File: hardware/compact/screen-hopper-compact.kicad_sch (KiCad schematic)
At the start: 11 parts, among them J1 USB_A_Host, J2 USB_C_Host, U1 6N137

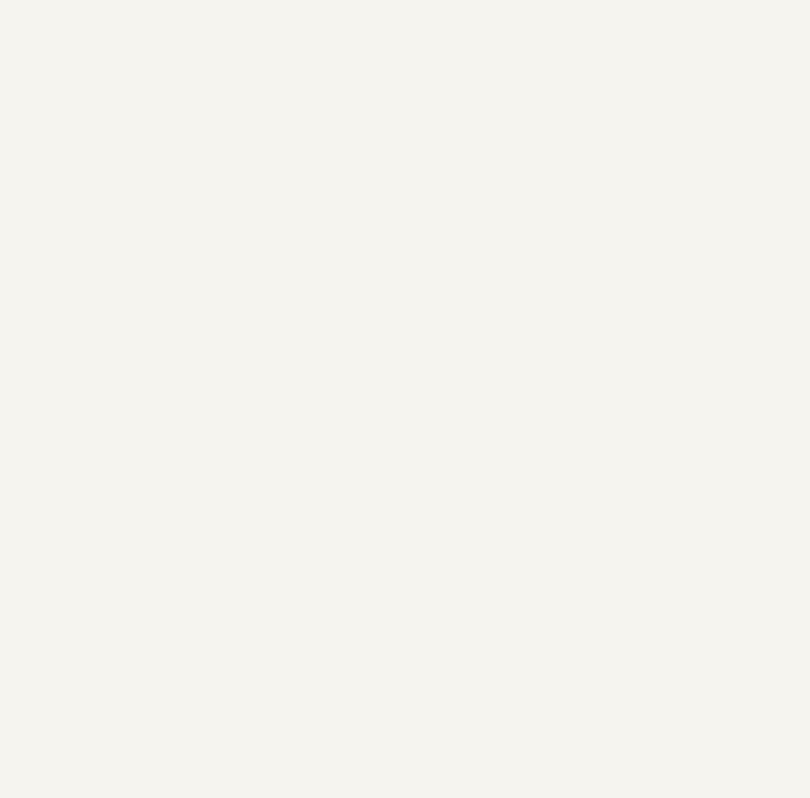
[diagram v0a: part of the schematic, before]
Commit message: feat: hardware board designs
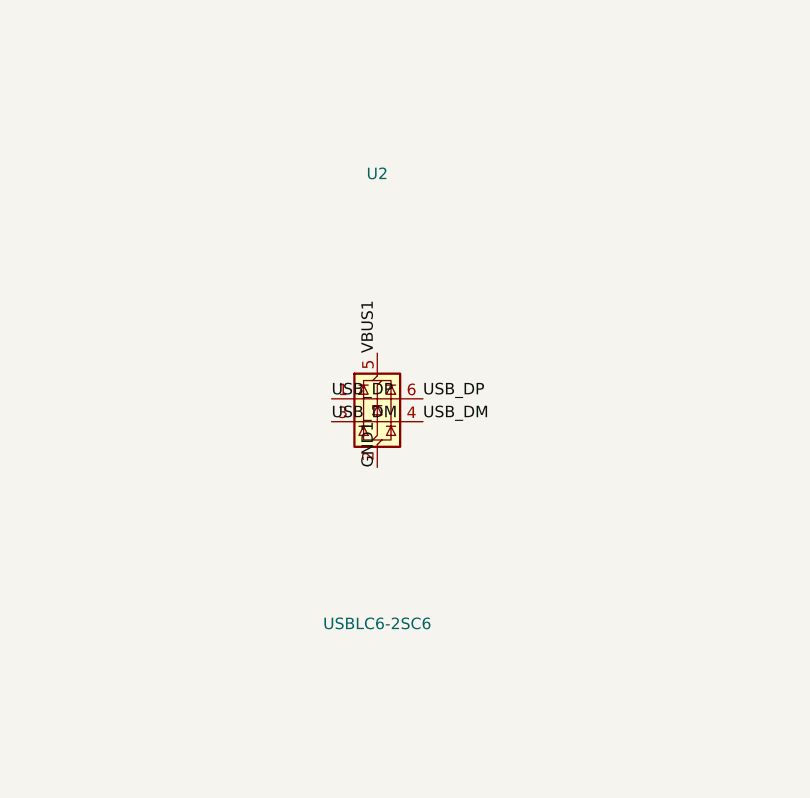
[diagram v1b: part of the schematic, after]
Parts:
- added U2: USBLC6-2SC6, Package_TO_SOT_SMD:SOT-23-6, symbol Power_Protection:USBLC6-2SC6
- J1: footprint Connector_USB:USB_A_Connfly_DS1095 -> Connector_USB:USB_A_TE_292303-7_Horizontal
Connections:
- net GND1: now also U2.2 (GND)
- net USB_DM: now also U2.3 (I/O2), U2.4 (I/O2)
- net USB_DP: now also U2.1 (I/O1), U2.6 (I/O1)
- net VBUS1: now also U2.5 (VBUS)
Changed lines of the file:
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@@
 		(instances
 			(project "screen-hopper"
-				(path "/1ca3d3a5-c661-41a7-ad19-cf03fba76b71"
+				(path "/e4afde65-c9ae-401d-b381-77b0abf5f55b"
 					(reference "A1")
 					(unit 1)
@@
 		(instances
 			(project "screen-hopper"
-				(path "/1ca3d3a5-c661-41a7-ad19-cf03fba76b71"
+				(path "/e4afde65-c9ae-401d-b381-77b0abf5f55b"
 					(reference "A2")
 					(unit 1)
@@
 		(instances
 			(project "screen-hopper"
-				(path "/1ca3d3a5-c661-41a7-ad19-cf03fba76b71"
+				(path "/e4afde65-c9ae-401d-b381-77b0abf5f55b"
 					(reference "A3")
 					(unit 1)
@@
 		(instances
 			(project "screen-hopper"
-				(path "/1ca3d3a5-c661-41a7-ad19-cf03fba76b71"
+				(path "/e4afde65-c9ae-401d-b381-77b0abf5f55b"
 					(reference "U1")
 					(unit 1)
@@
 		(instances
 			(project "screen-hopper"
-				(path "/1ca3d3a5-c661-41a7-ad19-cf03fba76b71"
+				(path "/e4afde65-c9ae-401d-b381-77b0abf5f55b"
 					(reference "R1")
 					(unit 1)
@@
 		(instances
 			(project "screen-hopper"
-				(path "/1ca3d3a5-c661-41a7-ad19-cf03fba76b71"
+				(path "/e4afde65-c9ae-401d-b381-77b0abf5f55b"
 					(reference "R2")
 					(unit 1)
@@
 		(instances
 			(project "screen-hopper"
-				(path "/1ca3d3a5-c661-41a7-ad19-cf03fba76b71"
+				(path "/e4afde65-c9ae-401d-b381-77b0abf5f55b"
 					(reference "C1")
 					(unit 1)
@@
 			(effects (font (size 1.27 1.27)))
 		)
-		(property "Footprint" "Connector_USB:USB_A_Connfly_DS1095"
+		(property "Footprint" "Connector_USB:USB_A_TE_292303-7_Horizontal"
 			(at 90.00 250.00 0)
 			(effects (font (size 1.27 1.27)) (hide yes))
@@
 		(instances
 			(project "screen-hopper"
-				(path "/1ca3d3a5-c661-41a7-ad19-cf03fba76b71"
+				(path "/e4afde65-c9ae-401d-b381-77b0abf5f55b"
 					(reference "J1")
 					(unit 1)
@@
 		(instances
 			(project "screen-hopper"
-				(path "/1ca3d3a5-c661-41a7-ad19-cf03fba76b71"
+				(path "/e4afde65-c9ae-401d-b381-77b0abf5f55b"
 					(reference "R3")
 					(unit 1)
@@
 		(instances
 			(project "screen-hopper"
-				(path "/1ca3d3a5-c661-41a7-ad19-cf03fba76b71"
+				(path "/e4afde65-c9ae-401d-b381-77b0abf5f55b"
 					(reference "R4")
 					(unit 1)
@@
 		(instances
 			(project "screen-hopper"
-				(path "/1ca3d3a5-c661-41a7-ad19-cf03fba76b71"
+				(path "/e4afde65-c9ae-401d-b381-77b0abf5f55b"
 					(reference "J2")
+					(unit 1)
+				)
+			)
+		)
+	)
+	(symbol
+		(lib_id "Power_Protection:USBLC6-2SC6")
+		(at 190.00 320.00 0)
+		(unit 1)
+		(exclude_from_sim no)
+		(in_bom yes)
+		(on_board yes)
+		(dnp no)
+		(property "Reference" "U2"
+			(at 190.00 295.00 0)
+			(effects (font (size 1.27 1.27)))
+		)
+		(property "Value" "USBLC6-2SC6"
+			(at 190.00 345.00 0)
+			(effects (font (size 1.27 1.27)))
+		)
+		(property "Footprint" "Package_TO_SOT_SMD:SOT-23-6"
+			(at 190.00 320.00 0)
+			(effects (font (size 1.27 1.27)) (hide yes))
+		)
+		(pin "1"
+		)
+		(pin "2"
+		)
+		(pin "3"
+		)
+		(pin "4"
+		)
+		(pin "5"
+		)
+		(pin "6"
+		)
+		(instances
+			(project "screen-hopper"
+				(path "/e4afde65-c9ae-401d-b381-77b0abf5f55b"
+					(reference "U2")
 					(unit 1)
 				)
@@
 		(effects (font (size 1.27 1.27)) (justify left bottom))
 	)
+	(label "VBUS1"
+		(at 190.00 314.92 270)
+		(effects (font (size 1.27 1.27)) (justify left bottom))
+	)
 	(label "GND1"
 		(at 190.00 195.56 90)
@@
 	(label "GND1"
 		(at 82.38 362.86 90)
+		(effects (font (size 1.27 1.27)) (justify left bottom))
+	)
+	(label "GND1"
+		(at 190.00 327.62 90)
 		(effects (font (size 1.27 1.27)) (justify left bottom))
 	)
@@
 		(effects (font (size 1.27 1.27)) (justify left bottom))
 	)
+	(label "USB_DM"
+		(at 184.92 322.54 0)
+		(effects (font (size 1.27 1.27)) (justify left bottom))
+	)
+	(label "USB_DM"
+		(at 195.08 322.54 180)
+		(effects (font (size 1.27 1.27)) (justify left bottom))
+	)
 	(label "USB_DP"
 		(at 97.62 250.00 180)
@@
 		(effects (font (size 1.27 1.27)) (justify left bottom))
 	)
+	(label "USB_DP"
+		(at 184.92 320.00 0)
+		(effects (font (size 1.27 1.27)) (justify left bottom))
+	)
+	(label "USB_DP"
+		(at 195.08 320.00 180)
+		(effects (font (size 1.27 1.27)) (justify left bottom))
+	)

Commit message: feat: hardware board designs
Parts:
- A1, A2, A3: MPN (none) -> SC1631; Manufacturer (none) -> Raspberry Pi
- J1: MPN (none) -> 292303-7; Manufacturer (none) -> TE Connectivity
- J2: MPN (none) -> TYPE-C-31-M-12; Manufacturer (none) -> HRO
- R1: MPN (none) -> RC0805JR-07470RL; Manufacturer (none) -> Yageo
- R2: MPN (none) -> RC0805FR-07680RL; Manufacturer (none) -> Yageo
- R3, R4: MPN (none) -> AC0805FR-0756KL; Manufacturer (none) -> Yageo
- U1: MPN (none) -> 6N137SM; Manufacturer (none) -> onsemi
- U2: MPN (none) -> USBLC6-2SC6; Manufacturer (none) -> STMicroelectronics
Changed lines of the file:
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@@
+			(effects (font (size 1.27 1.27)) (hide yes))
+		)
+		(property "MPN" "SC1631"
+			(at 190.00 160.00 0)
+			(effects (font (size 1.27 1.27)) (hide yes))
+		)
+		(property "Manufacturer" "Raspberry Pi"
+			(at 190.00 160.00 0)
 			(effects (font (size 1.27 1.27)) (hide yes))
 		)
@@
 		(instances
 			(project "screen-hopper"
-				(path "/546f9845-45df-437b-a8f0-1d6148817de3"
+				(path "/468433d7-c8e3-4031-b0d4-1b453175f0b2"
 					(reference "A1")
 					(unit 1)
@@
 			(effects (font (size 1.27 1.27)) (hide yes))
 		)
+		(property "MPN" "SC1631"
+			(at 90.00 160.00 0)
+			(effects (font (size 1.27 1.27)) (hide yes))
+		)
+		(property "Manufacturer" "Raspberry Pi"
+			(at 90.00 160.00 0)
+			(effects (font (size 1.27 1.27)) (hide yes))
+		)
 		(pin "1"
 		)
@@
 		(instances
 			(project "screen-hopper"
-				(path "/546f9845-45df-437b-a8f0-1d6148817de3"
+				(path "/468433d7-c8e3-4031-b0d4-1b453175f0b2"
 					(reference "A2")
 					(unit 1)
@@
 			(effects (font (size 1.27 1.27)) (hide yes))
 		)
+		(property "MPN" "SC1631"
+			(at 290.00 160.00 0)
+			(effects (font (size 1.27 1.27)) (hide yes))
+		)
+		(property "Manufacturer" "Raspberry Pi"
+			(at 290.00 160.00 0)
+			(effects (font (size 1.27 1.27)) (hide yes))
+		)
 		(pin "1"
 		)
@@
 		(instances
 			(project "screen-hopper"
-				(path "/546f9845-45df-437b-a8f0-1d6148817de3"
+				(path "/468433d7-c8e3-4031-b0d4-1b453175f0b2"
 					(reference "A3")
 					(unit 1)
@@
 			(effects (font (size 1.27 1.27)) (hide yes))
 		)
+		(property "MPN" "6N137SM"
+			(at 185.00 70.00 0)
+			(effects (font (size 1.27 1.27)) (hide yes))
+		)
+		(property "Manufacturer" "onsemi"
+			(at 185.00 70.00 0)
+			(effects (font (size 1.27 1.27)) (hide yes))
+		)
 		(pin "1"
 		)
@@
 		(instances
 			(project "screen-hopper"
-				(path "/546f9845-45df-437b-a8f0-1d6148817de3"
+				(path "/468433d7-c8e3-4031-b0d4-1b453175f0b2"
 					(reference "U1")
 					(unit 1)
@@
 			(effects (font (size 1.27 1.27)) (hide yes))
 		)
-		(pin "1"
-		)
-		(pin "2"
-		)
-		(instances
-			(project "screen-hopper"
-				(path "/546f9845-45df-437b-a8f0-1d6148817de3"
+		(property "MPN" "RC0805JR-07470RL"
+			(at 130.00 70.00 0)
+			(effects (font (size 1.27 1.27)) (hide yes))
+		)
+		(property "Manufacturer" "Yageo"
+			(at 130.00 70.00 0)
+			(effects (font (size 1.27 1.27)) (hide yes))
+		)
+		(pin "1"
+		)
+		(pin "2"
+		)
+		(instances
+			(project "screen-hopper"
+				(path "/468433d7-c8e3-4031-b0d4-1b453175f0b2"
 					(reference "R1")
 					(unit 1)
@@
 			(effects (font (size 1.27 1.27)) (hide yes))
 		)
-		(pin "1"
-		)
-		(pin "2"
-		)
-		(instances
-			(project "screen-hopper"
-				(path "/546f9845-45df-437b-a8f0-1d6148817de3"
+		(property "MPN" "RC0805FR-07680RL"
+			(at 240.00 60.00 0)
+			(effects (font (size 1.27 1.27)) (hide yes))
+		)
+		(property "Manufacturer" "Yageo"
+			(at 240.00 60.00 0)
+			(effects (font (size 1.27 1.27)) (hide yes))
+		)
+		(pin "1"
+		)
+		(pin "2"
+		)
+		(instances
+			(project "screen-hopper"
+				(path "/468433d7-c8e3-4031-b0d4-1b453175f0b2"
 					(reference "R2")
 					(unit 1)
@@
 		(instances
 			(project "screen-hopper"
-				(path "/546f9845-45df-437b-a8f0-1d6148817de3"
+				(path "/468433d7-c8e3-4031-b0d4-1b453175f0b2"
 					(reference "C1")
 					(unit 1)
@@
 			(effects (font (size 1.27 1.27)) (hide yes))
 		)
+		(property "MPN" "292303-7"
+			(at 90.00 250.00 0)
+			(effects (font (size 1.27 1.27)) (hide yes))
+		)
+		(property "Manufacturer" "TE Connectivity"
+			(at 90.00 250.00 0)
+			(effects (font (size 1.27 1.27)) (hide yes))
+		)
 		(pin "1"
 		)
@@
 		(instances
 			(project "screen-hopper"
-				(path "/546f9845-45df-437b-a8f0-1d6148817de3"
+				(path "/468433d7-c8e3-4031-b0d4-1b453175f0b2"
 					(reference "J1")
 					(unit 1)
@@
 			(effects (font (size 1.27 1.27)) (hide yes))
 		)
-		(pin "1"
-		)
-		(pin "2"
-		)
-		(instances
-			(project "screen-hopper"
-				(path "/546f9845-45df-437b-a8f0-1d6148817de3"
+		(property "MPN" "AC0805FR-0756KL"
+			(at 30.00 300.00 0)
+			(effects (font (size 1.27 1.27)) (hide yes))
+		)
+		(property "Manufacturer" "Yageo"
+			(at 30.00 300.00 0)
+			(effects (font (size 1.27 1.27)) (hide yes))
+		)
+		(pin "1"
+		)
+		(pin "2"
+		)
+		(instances
+			(project "screen-hopper"
+				(path "/468433d7-c8e3-4031-b0d4-1b453175f0b2"
 					(reference "R3")
 					(unit 1)
@@
 			(effects (font (size 1.27 1.27)) (hide yes))
 		)
-		(pin "1"
-		)
-		(pin "2"
-		)
-		(instances
-			(project "screen-hopper"
-				(path "/546f9845-45df-437b-a8f0-1d6148817de3"
+		(property "MPN" "AC0805FR-0756KL"
+			(at 30.00 340.00 0)
+			(effects (font (size 1.27 1.27)) (hide yes))
+		)
+		(property "Manufacturer" "Yageo"
+			(at 30.00 340.00 0)
+			(effects (font (size 1.27 1.27)) (hide yes))
+		)
+		(pin "1"
+		)
+		(pin "2"
+		)
+		(instances
+			(project "screen-hopper"
+				(path "/468433d7-c8e3-4031-b0d4-1b453175f0b2"
 					(reference "R4")
 					(unit 1)
@@
 			(effects (font (size 1.27 1.27)) (hide yes))
 		)
+		(property "MPN" "TYPE-C-31-M-12"
+			(at 90.00 340.00 0)
+			(effects (font (size 1.27 1.27)) (hide yes))
+		)
+		(property "Manufacturer" "HRO"
+			(at 90.00 340.00 0)
+			(effects (font (size 1.27 1.27)) (hide yes))
+		)
 		(pin "A1"
 		)
@@
 		(instances
 			(project "screen-hopper"
-				(path "/546f9845-45df-437b-a8f0-1d6148817de3"
+				(path "/468433d7-c8e3-4031-b0d4-1b453175f0b2"
 					(reference "J2")
 					(unit 1)
@@
 			(effects (font (size 1.27 1.27)) (hide yes))
 		)
+		(property "MPN" "USBLC6-2SC6"
+			(at 190.00 320.00 0)
+			(effects (font (size 1.27 1.27)) (hide yes))
+		)
+		(property "Manufacturer" "STMicroelectronics"
+			(at 190.00 320.00 0)
+			(effects (font (size 1.27 1.27)) (hide yes))
+		)
 		(pin "1"
 		)
@@
 		(instances
 			(project "screen-hopper"
-				(path "/546f9845-45df-437b-a8f0-1d6148817de3"
+				(path "/468433d7-c8e3-4031-b0d4-1b453175f0b2"
 					(reference "U2")
 					(unit 1)
